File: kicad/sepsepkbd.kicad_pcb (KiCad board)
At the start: 2 copper layers, 202.9 x 111.3 mm, 47 parts, among them J1 MJ-4PP-9, J2 Conn_01x04_Socket, J3 Conn_01x04_Socket, SW1 SW_PUSH, SW10 SW_PUSH, SW11 SW_PUSH, SW12 SW_PUSH, SW13 SW_PUSH, SW14 SW_PUSH, SW15 SW_PUSH, SW16 SW_PUSH, SW17 SW_PUSH, SW18 SW_PUSH, SW19 SW_PUSH, SW2 SW_PUSH, SW20 SW_PUSH, SW21 SW_PUSH, SW3 SW_PUSH, SW4 SW_PUSH, SW5 SW_PUSH, SW6 SW_PUSH, SW7 SW_PUSH, SW8 SW_PUSH, SW9 SW_PUSH, U1 ProMicro

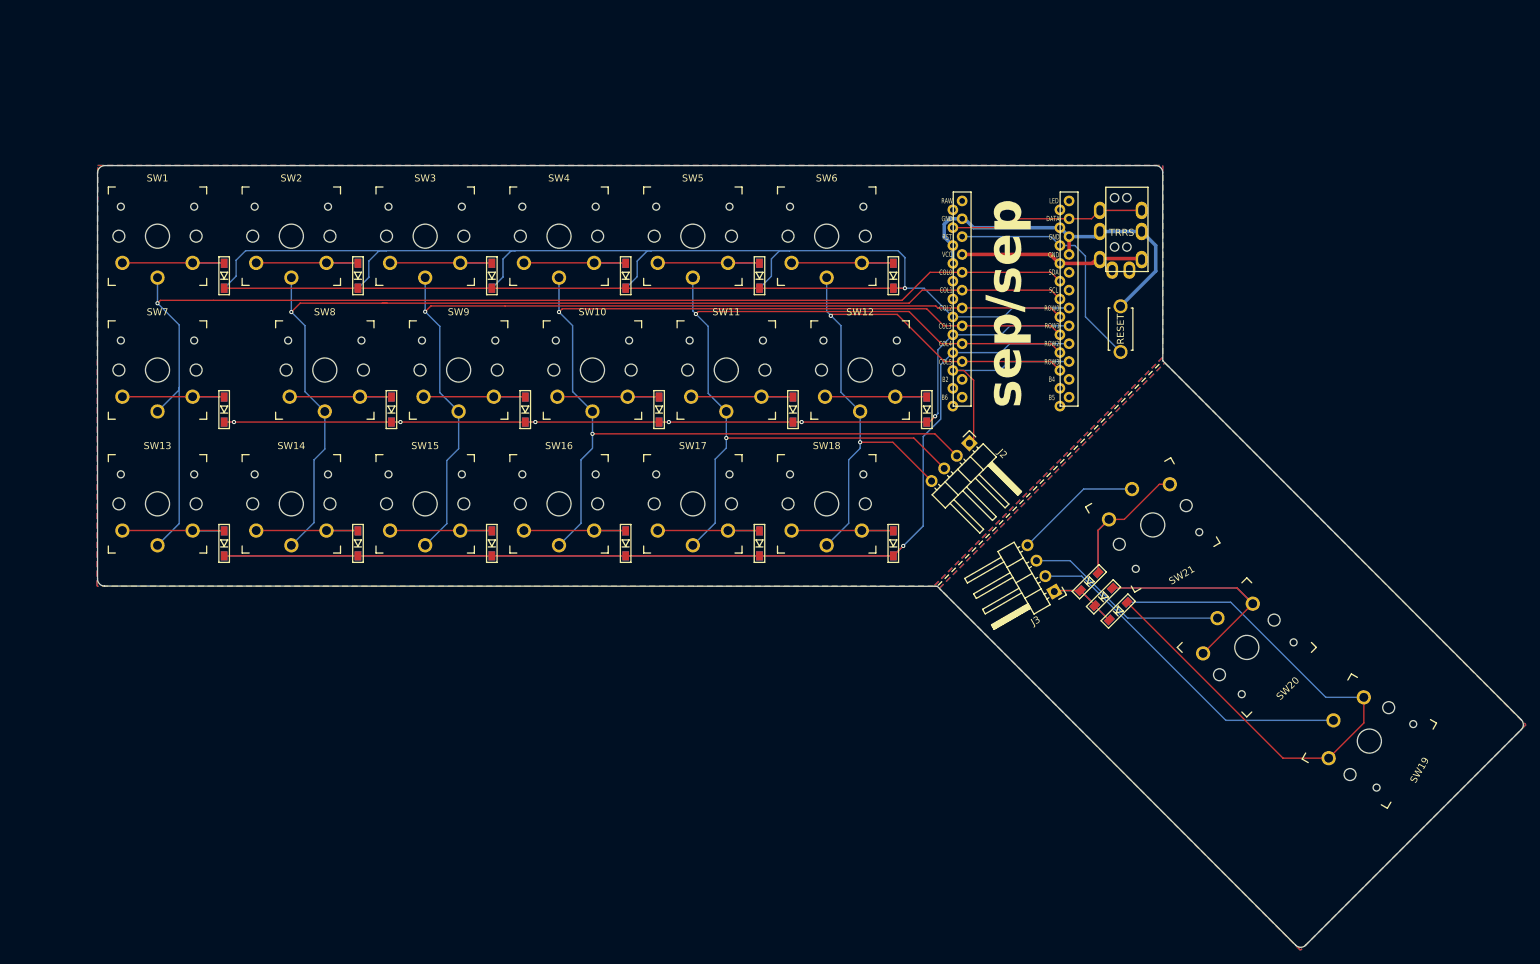
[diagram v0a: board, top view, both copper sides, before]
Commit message: 2.1
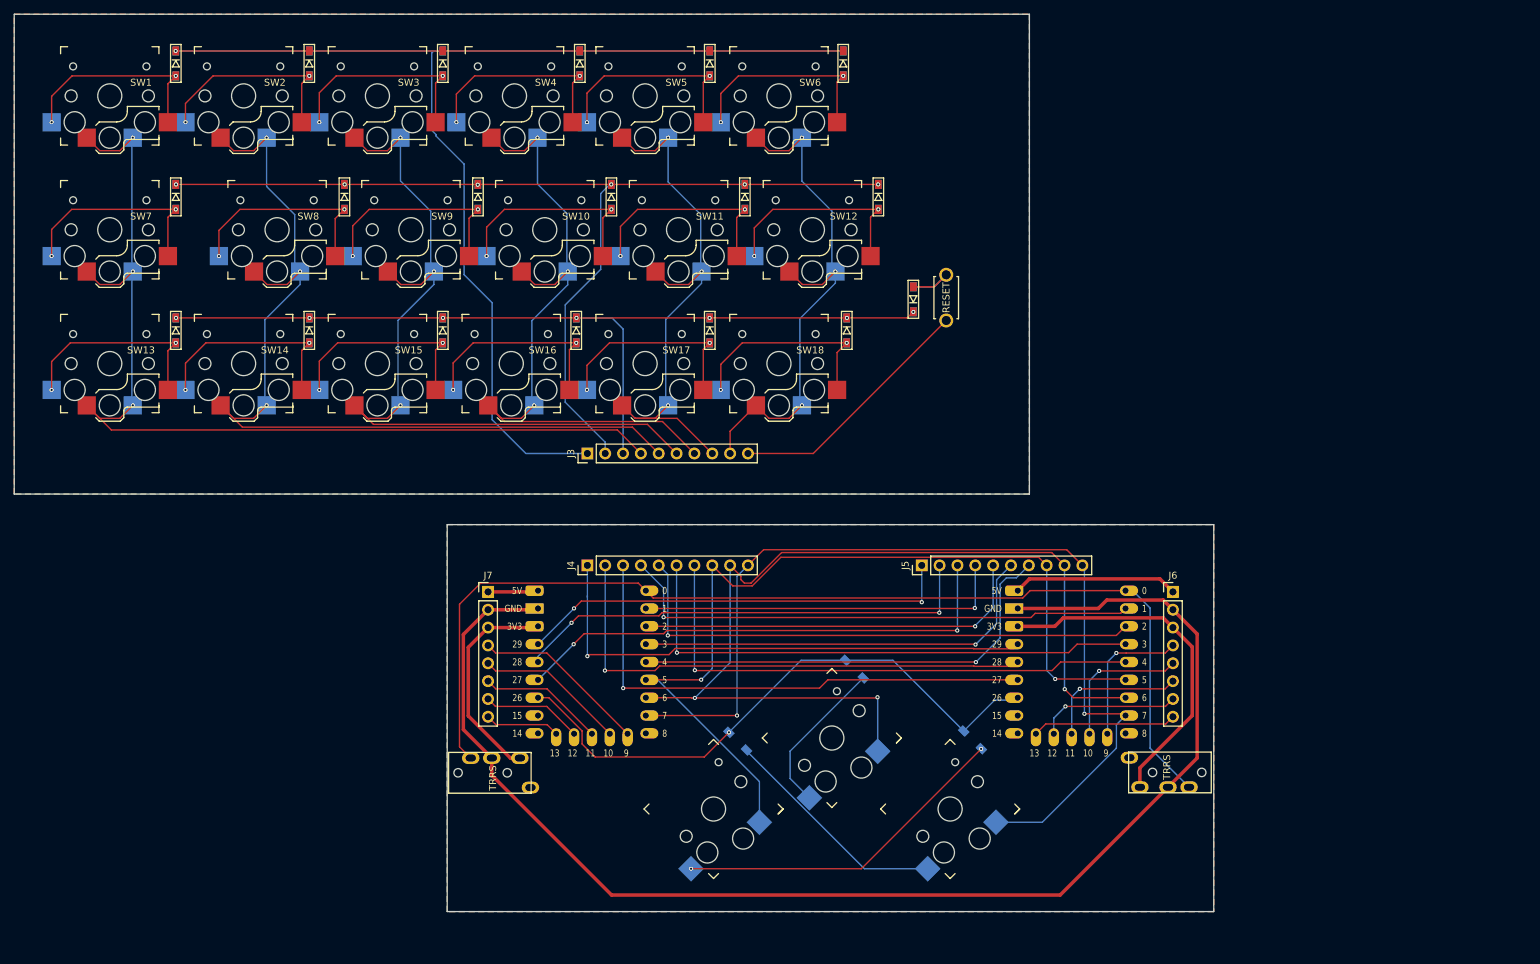
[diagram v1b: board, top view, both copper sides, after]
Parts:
- removed SW_RESET1: SW_PUSH, kbd:ResetSW
- added D22: D, kbd:D3_SMD_v2, B.Cu at (118.4, 118.9)
- added J4: Conn_01x10_Pin, Connector_PinHeader_2.54mm:PinHeader_1x10_P2.54mm_Vertical, F.Cu at (97.0, 93.9)
- added J5: Conn_01x10_Pin, Connector_PinHeader_2.54mm:PinHeader_1x10_P2.54mm_Vertical, F.Cu at (144.6, 93.9)
- added J6: Conn_01x08_Pin, Connector_PinHeader_2.54mm:PinHeader_1x08_P2.54mm_Vertical, F.Cu at (180.3, 97.7)
- added J7: Conn_01x08_Pin, Connector_PinHeader_2.54mm:PinHeader_1x08_P2.54mm_Vertical, F.Cu at (82.9, 97.7)
- added SW22: SW_PUSH, keyswitches:Kailh_socket_PG1350, F.Cu at (148.6, 128.6)
- added U2: RP2040-Zero, isw-kbd:RP2040-Zero-THT, F.Cu at (97.7, 107.7)
- D20, D21: footprint kbd:D3_SMD -> kbd:D3_SMD_v2; moved to B.Cu
- J1: footprint kbd:MJ-4PP-9 -> kbd:MJ-4PP-9_1side
- J2: value Conn_01x04_Socket -> MJ-4PP-9; footprint Connector_PinHeader_2.54mm:PinHeader_1x04_P2.54mm_Horizontal -> kbd:MJ-4PP-9_1side
- J3: value Conn_01x04_Socket -> Conn_01x10_Pin; footprint Connector_PinHeader_2.54mm:PinHeader_1x04_P2.54mm_Horizontal -> Connector_PinHeader_2.54mm:PinHeader_1x10_P2.54mm_Vertical
- SW1, SW10, SW11, SW12, SW13, SW14, SW15, SW16, SW17, SW18, SW2, SW3, SW4, SW5, SW6, SW7, SW8, SW9: footprint keyswitches:SW_PG1350_reversible -> keyswitches:Kailh_socket_PG1350_reversible
- SW19: footprint keyswitches:SW_PG1350_reversible -> kbd:ResetSW
- SW20, SW21: footprint keyswitches:SW_PG1350_reversible -> keyswitches:Kailh_socket_PG1350
- U1: value ProMicro -> RP2040-Zero; footprint kbd:ProMicro_v2 -> isw-kbd:RP2040-Zero-THT
- moved J2 87.9 mm to (77.1, 123.5), turned to 90 degrees
- moved SW19 87.2 mm to (148.1, 55.8), turned to -90 degrees
- moved J1 84.2 mm to (185.9, 123.4), turned to -90 degrees
- moved SW20 79.3 mm to (115.0, 128.6), turned to 45 degrees
- moved J3 69.3 mm to (97.0, 78.0), turned to 90 degrees
- moved SW21 54.8 mm to (131.8, 118.5), turned to 45 degrees
- moved D19 53.1 mm to (143.4, 56.0), turned to 90 degrees
- moved U1 51.8 mm to (165.9, 107.7)
- moved D21 35.7 mm to (135.0, 108.7), turned to -45 degrees
- moved D17 31.1 mm to (114.4, 60.5), turned to -90 degrees
- moved D16 31.1 mm to (95.4, 60.5), turned to -90 degrees
- moved D15 31.1 mm to (76.4, 60.5), turned to -90 degrees
- moved D14 31.1 mm to (57.4, 60.5), turned to -90 degrees
- moved D13 31.1 mm to (38.4, 60.5), turned to -90 degrees
- moved D6 31.1 mm to (133.4, 22.5), turned to -90 degrees
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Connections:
- D1 pad 1: row0 -> /t_row0
- D10 pad 1: row1 -> /t_row1
- D11 pad 1: row1 -> /t_row1
- D12 pad 1: row1 -> /t_row1
- D13 pad 1: row2 -> /t_row2
- D14 pad 1: row2 -> /t_row2
- D15 pad 1: row2 -> /t_row2
- D16 pad 1: row2 -> /t_row2
- D17 pad 1: row2 -> /t_row2
- D18 pad 1: row2 -> /t_row2
- D19 pad 1: Net-(D19-K) -> /t_row2
- D2 pad 1: row0 -> /t_row0
- D20 pad 1: Net-(D19-K) -> bu1_row3
- D21 pad 1: Net-(D19-K) -> bu1_row3
- D3 pad 1: row0 -> /t_row0
- D4 pad 1: row0 -> /t_row0
- D5 pad 1: row0 -> /t_row0
- D6 pad 1: row0 -> /t_row0
- D7 pad 1: row1 -> /t_row1
- D8 pad 1: row1 -> /t_row1
- D9 pad 1: row1 -> /t_row1
- J1 pad D: VCC -> u1_3.3v
- J3 pad 1: Net-(D19-K) -> /t_row0
- J3 pad 2: Net-(J3-Pin_2) -> /t_row1
- J3 pad 3: Net-(J3-Pin_3) -> /t_row2
- J3 pad 4: Net-(J3-Pin_4) -> /t_col0
- SW1 pad 1: col0 -> /t_col0
- SW10 pad 1: col3 -> /t_col3
- SW11 pad 1: col4 -> /t_col4
- SW12 pad 1: col5 -> /t_col5
- SW13 pad 1: col0 -> /t_col0
- SW14 pad 1: col1 -> /t_col1
- SW15 pad 1: col2 -> /t_col2
- SW16 pad 1: col3 -> /t_col3
- SW17 pad 1: col4 -> /t_col4
- SW18 pad 1: col5 -> /t_col5
- SW19 pad 1: Net-(J3-Pin_2) -> /t_col6
- SW2 pad 1: col1 -> /t_col1
- SW20 pad 1: Net-(J3-Pin_3) -> bu1_col4
- SW21 pad 1: Net-(J3-Pin_4) -> bu1_col5
- SW3 pad 1: col2 -> /t_col2
- SW4 pad 1: col3 -> /t_col3
- SW5 pad 1: col4 -> /t_col4
- SW6 pad 1: col5 -> /t_col5
- SW7 pad 1: col0 -> /t_col0
- SW8 pad 1: col1 -> /t_col1
- SW9 pad 1: col2 -> /t_col2
- U1 pad 1: unconnected-(U1-TX0/D3-Pad1)_0 -> bu1_col0
- U1 pad 10: row3 -> bu1_op2
- U1 pad 11: unconnected-(U1-8/B4-Pad11)_0 -> bu1_op3
- U1 pad 12: unconnected-(U1-9/B5-Pad12) -> bu1_op4
- U1 pad 13: unconnected-(U1-B6/10-Pad13) -> bu1_op5
- U1 pad 15: col5 -> unconnected-(U1-Pad15)
- U1 pad 2: data -> bu1_col1
- U1 pad 3: GND -> bu1_col2
- U1 pad 4: GND -> bu1_col3
- U1 pad 5: unconnected-(U1-2/D1/SDA-Pad5) -> bu1_col4
- U1 pad 6: unconnected-(U1-3/D0/SCL-Pad6) -> bu1_col5
- U1 pad 7: row0 -> bu1_col6
- U1 pad 8: row1 -> unconnected-(U1-Pad8)
- U1 pad 9: row2 -> bu1_op1
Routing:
- net /t_row0: track 0.00 -> 263.0 mm, vias 0 -> 1
- net row0: track 259.1 -> 0.00 mm, vias 1 -> 0
- net row2: track 242.0 -> 0.00 mm, vias 1 -> 0
- net col0: track 176.2 -> 0.00 mm, vias 1 -> 0
- net col3: track 168.2 -> 0.00 mm, vias 2 -> 0
- net col1: track 154.0 -> 0.00 mm, vias 1 -> 0
- net /t_col0: track 0.00 -> 144.3 mm, vias 0 -> 3
- net /t_row1: track 0.00 -> 143.5 mm, vias 0 -> 6
- net GND: track 51.9 -> 195.1 mm
- net bu1_col5: track 0.00 -> 140.0 mm, vias 0 -> 3
- net row1: track 139.5 -> 0.00 mm, vias 6 -> 0
- net bu1_col6: track 0.00 -> 138.3 mm, vias 0 -> 2
- net col2: track 133.4 -> 0.00 mm, vias 1 -> 0
- net /t_col1: track 0.00 -> 131.7 mm, vias 0 -> 3
- net bu1_col4: track 0.00 -> 130.5 mm, vias 0 -> 2
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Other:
- board size 202.9 x 111.3 mm -> 170.7 x 127.7 mm
- board text removed: "sep/sep"
